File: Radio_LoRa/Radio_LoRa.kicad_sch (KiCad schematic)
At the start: 4 parts, among them J1 SMA-J-P-H-ST-EM1, J2 M80-8770405, J3 M80-8770405, U1 RFM95W-915S2

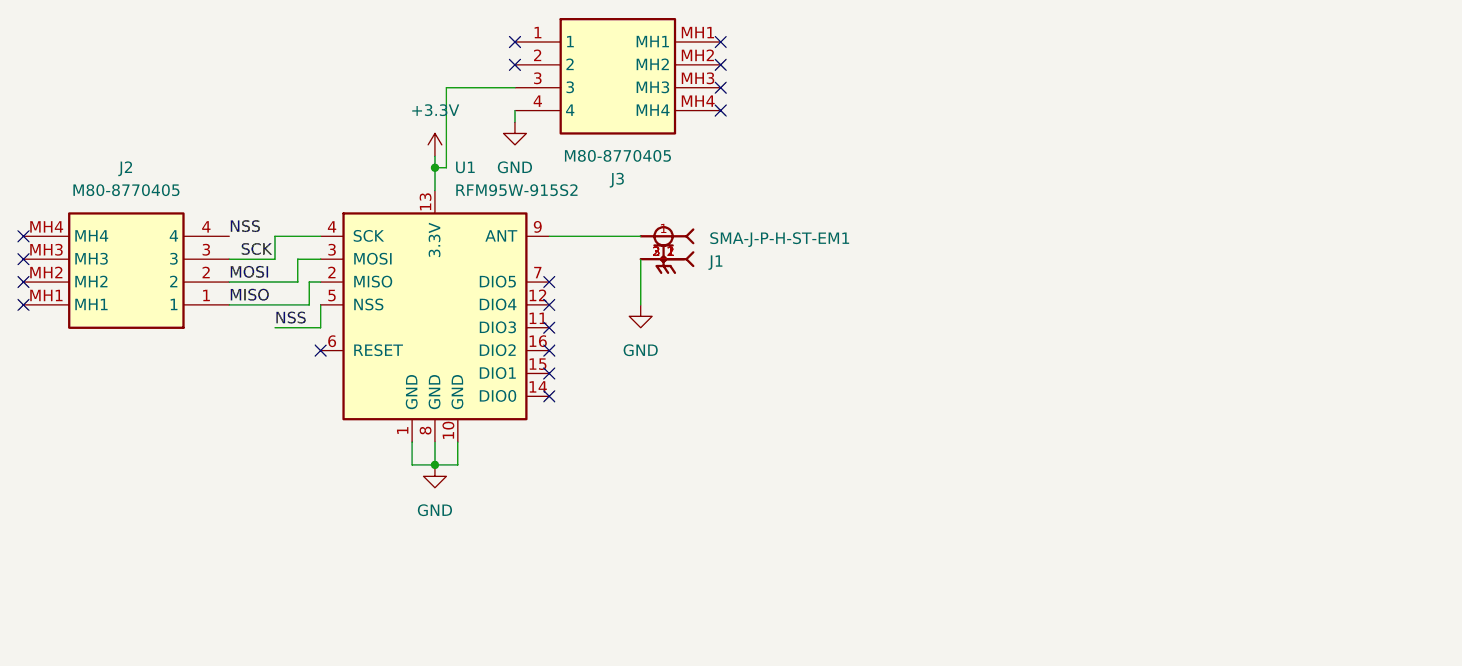
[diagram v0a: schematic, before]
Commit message: LC24 PCBs
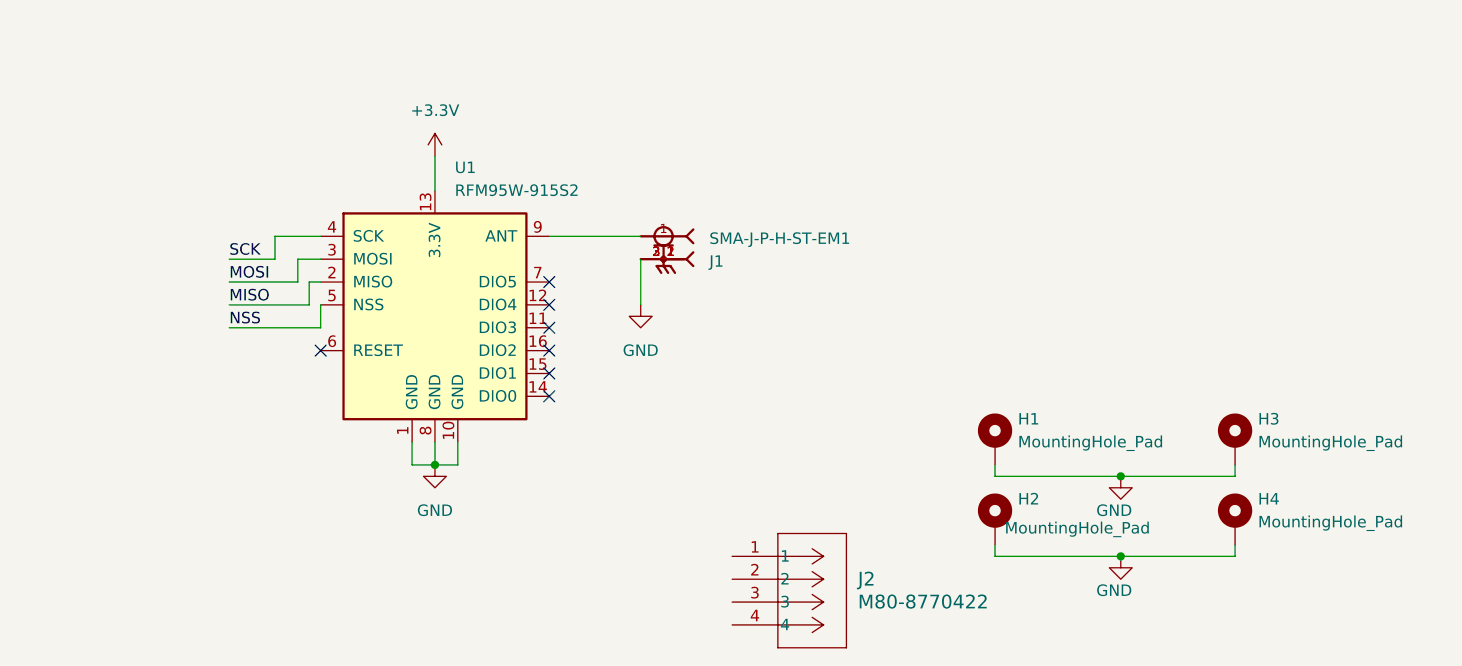
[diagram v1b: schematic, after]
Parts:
- removed J2, J3: M80-8770405, M808770405, symbol M80-8770405:M80-8770405
- added H1, H2, H3, H4: MountingHole_Pad, Mounting_Wuerth:Mounting_Wuerth_WA-SMSI-M1.6_H1mm_9774010633, symbol Mechanical:MountingHole_Pad
- added J2: M80-8770422, Harwin-M80-8770422:CONN_M80-87704_HRW, symbol Harwin-M80-8770422:M80-8770422
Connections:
- net GND: now also H1.1, H2.1, H3.1, H4.1
- no-connect marks 17 -> 7
